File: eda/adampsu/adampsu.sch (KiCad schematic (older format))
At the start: 56 parts, among them J1 Barrel_Jack_Switch, J2 Conn_2Rows-09Pins, J3 DB9_Female, Q1 BUK7880-55A_CUX, SW1 30V 300mA Latching Switch, U1 TPS561201, U2 TPS54531DDAR

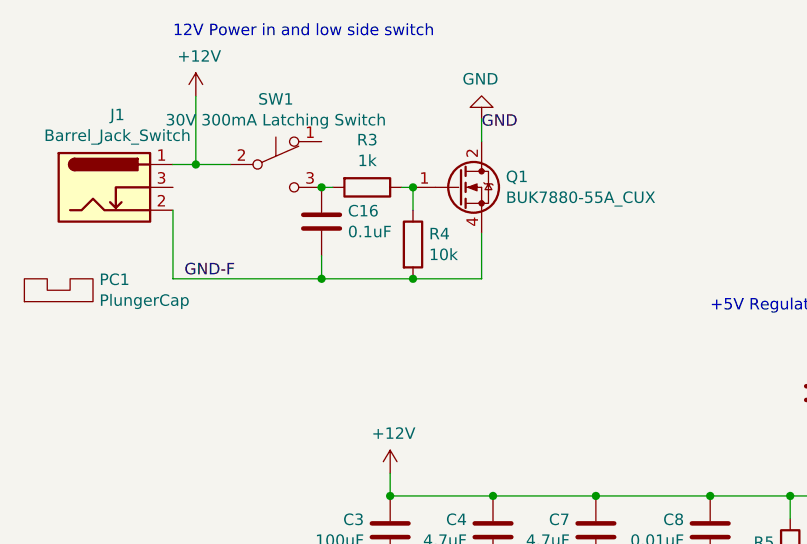
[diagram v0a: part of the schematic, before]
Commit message: Export schematic and PCB to PDFs
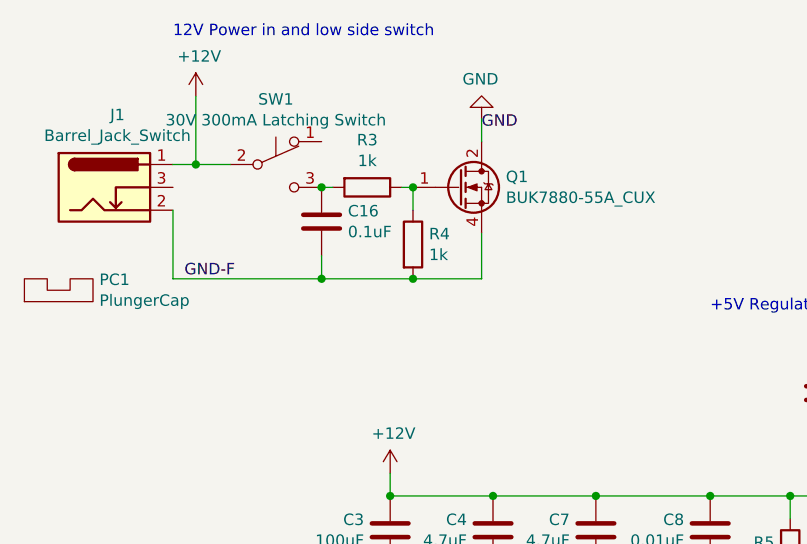
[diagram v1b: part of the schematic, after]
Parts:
- R4: value 10k -> 1k; dk 311-10KGRCT-ND -> 311-1.0KGRCT-ND; mfr RC0603JR-0710KL -> RC0603JR-071KL; mouser 603-RC0603JR-0710KL -> 603-RC0603JR-071KL
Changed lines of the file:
@@
 Wire Wire Line
 	2250 1500 2300 1500
-$Comp
-L Device:R R4
-U 1 1 5DBAB23A
-P 2300 1750
-F 0 "R4" H 2370 1796 50  0000 L CNN
-F 1 "10k" H 2370 1705 50  0000 L CNN
-F 2 "Resistor_SMD:R_0603_1608Metric_Pad1.05x0.95mm_HandSolder" V 2230 1750 50  0001 C CNN
-F 3 "http://www.yageo.com/documents/recent/PYu-RC_Group_51_RoHS_L_10.pdf" H 2300 1750 50  0001 C CNN
-F 4 "311-10KGRCT-ND" H 2300 1750 50  0001 C CNN "dk"
-F 5 "RC0603JR-0710KL" H 2300 1750 50  0001 C CNN "mfr"
-F 6 "603-RC0603JR-0710KL" H 2300 1750 50  0001 C CNN "mouser"
-	1    2300 1750
-	1    0    0    -1
-$EndComp
 Wire Wire Line
 	2300 1500 2300 1600
@@
 	2600 1700 2600 1900
 Wire Wire Line
-	2600 1900 2300 1900
-Wire Wire Line
-	2300 1900 1900 1900
-Wire Wire Line
 	1250 1900 1250 1600
-Connection ~ 2300 1900
 Text Label 1300 1900 0    50   ~ 0
 GND-F
@@
 	0    1    1    0
 $EndComp
+$Comp
+L Device:R R4
+U 1 1 5DCAA07F
+P 2300 1750
+F 0 "R4" H 2370 1796 50  0000 L CNN
+F 1 "1k" H 2370 1705 50  0000 L CNN
+F 2 "Resistor_SMD:R_0603_1608Metric_Pad1.05x0.95mm_HandSolder" V 2230 1750 50  0001 C CNN
+F 3 "http://www.yageo.com/documents/recent/PYu-RC_Group_51_RoHS_L_10.pdf" H 2300 1750 50  0001 C CNN
+F 4 "311-1.0KGRCT-ND" H 2300 1750 50  0001 C CNN "dk"
+F 5 "RC0603JR-071KL" H 2300 1750 50  0001 C CNN "mfr"
+F 6 "603-RC0603JR-071KL" H 2300 1750 50  0001 C CNN "mouser"
+	1    2300 1750
+	1    0    0    -1
+$EndComp
+Wire Wire Line
+	1900 1900 2300 1900
+Connection ~ 2300 1900
+Wire Wire Line
+	2300 1900 2600 1900
 $EndSCHEMATC
